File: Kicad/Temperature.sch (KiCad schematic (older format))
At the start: 2 parts

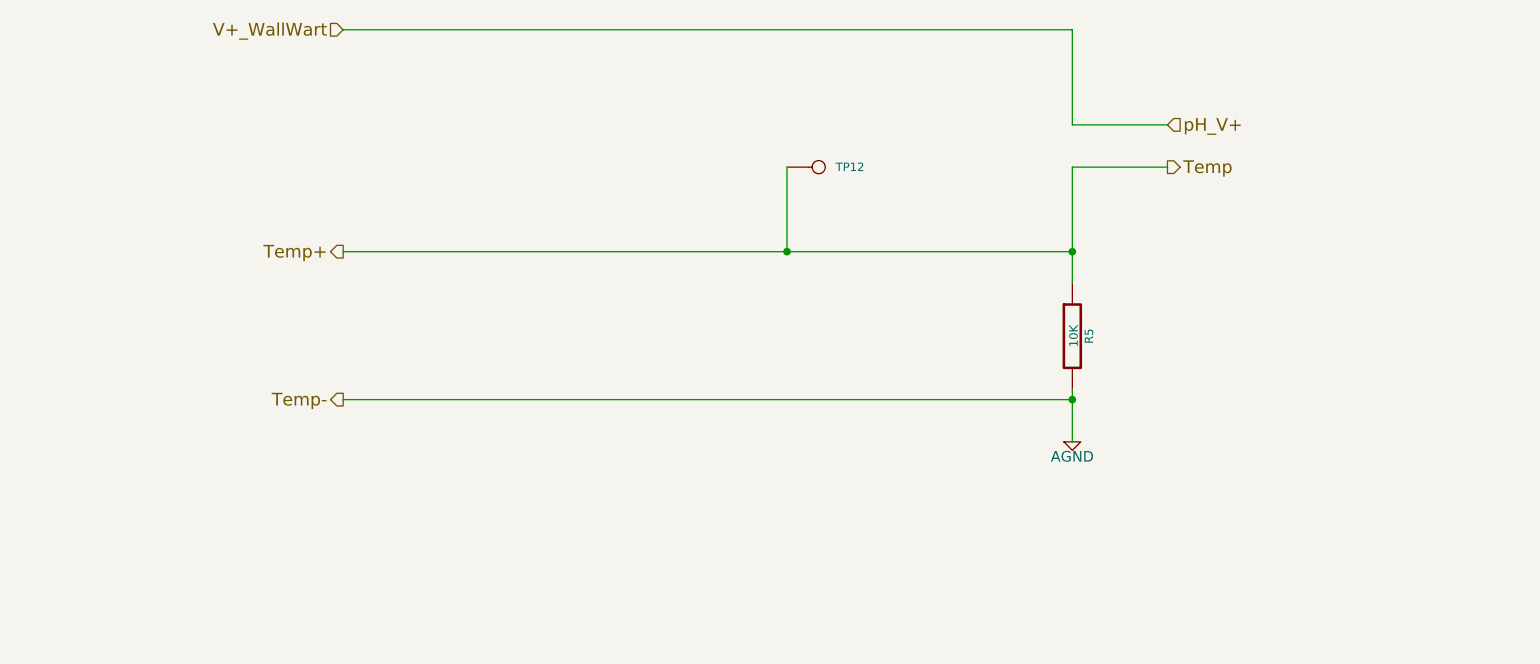
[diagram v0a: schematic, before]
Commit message: updates for dev rev 2
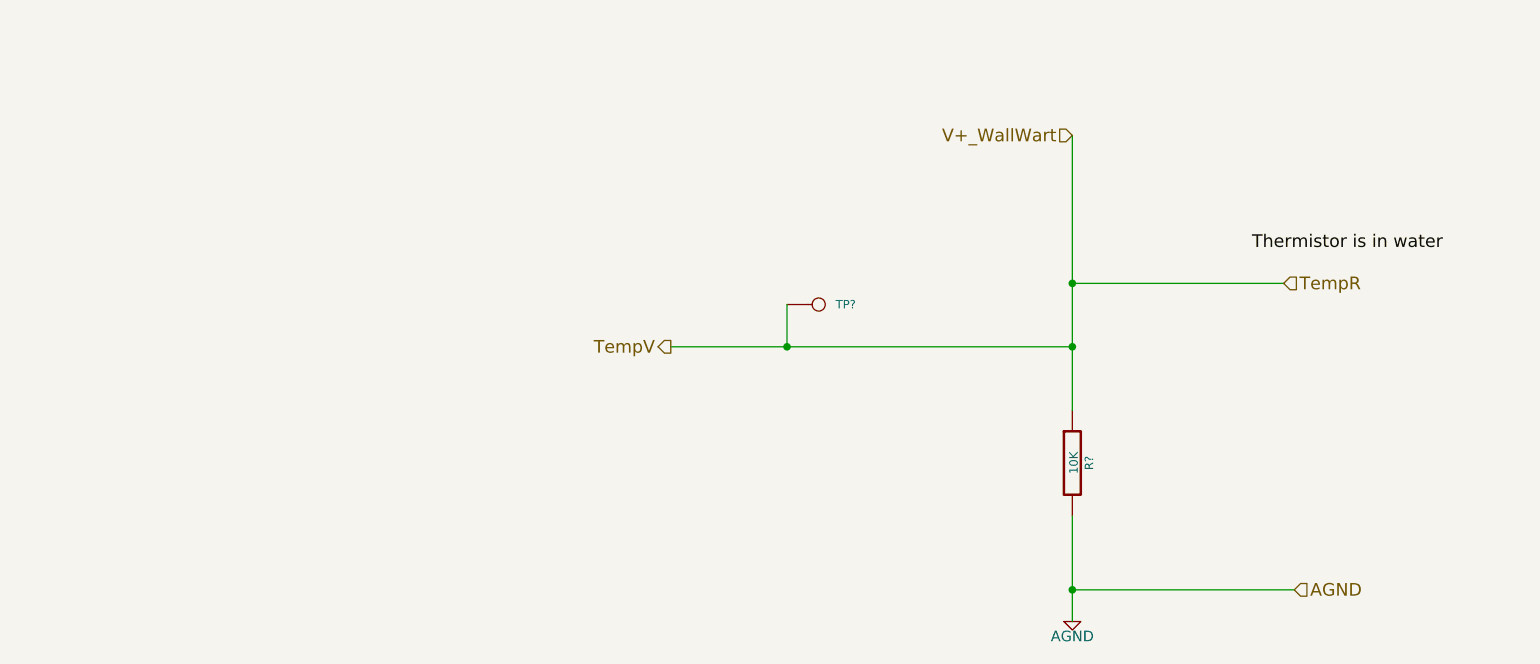
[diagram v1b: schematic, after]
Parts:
- removed R5: 10K, ~, symbol R
- removed TP12: CONN_1, symbol CONN_1
- added R?: 10K, ~, symbol R
- added TP?: CONN_1, symbol CONN_1
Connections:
- net AGND: now also R?.2
- new net TempR: R?.1, TP?.1
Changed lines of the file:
@@
 Sheet 6 7
 Title ""
-Date "21 aug 2014"
+Date "9 sep 2014"
 Rev ""
 Comp ""
@@
 Comment4 ""
 $EndDescr
-Text HLabel 1950 1500 0    60   Input ~ 0
+Text HLabel 5400 2000 0    60   Input ~ 0
 V+_WallWart
-Wire Wire Line
-	1950 1500 5400 1500
 $Comp
 L AGND #PWR012
 U 1 1 53CE414D
-P 5400 3450
-F 0 "#PWR012" H 5400 3450 40  0001 C CNN
-F 1 "AGND" H 5400 3380 50  0000 C CNN
-F 2 "" H 5400 3450 60  0000 C CNN
-F 3 "" H 5400 3450 60  0000 C CNN
-	1    5400 3450
+P 5400 4300
+F 0 "#PWR012" H 5400 4300 40  0001 C CNN
+F 1 "AGND" H 5400 4230 50  0000 C CNN
+F 2 "" H 5400 4300 60  0000 C CNN
+F 3 "" H 5400 4300 60  0000 C CNN
+	1    5400 4300
+	1    0    0    -1
+$EndComp
+$Comp
+L R R?
+U 1 1 540DEB6D
+P 5400 3550
+F 0 "R?" V 5480 3550 40  0000 C CNN
+F 1 "10K" V 5407 3551 40  0000 C CNN
+F 2 "~" V 5330 3550 30  0000 C CNN
+F 3 "~" H 5400 3550 30  0000 C CNN
+	1    5400 3550
+	1    0    0    -1
+$EndComp
+Text HLabel 6400 2700 2    60   Input ~ 0
+TempR
+Text HLabel 3500 3000 0    60   Output ~ 0
+TempV
+Text HLabel 6450 4150 2    60   Input ~ 0
+AGND
+$Comp
+L CONN_1 TP?
+U 1 1 540E05A9
+P 4200 2800
+F 0 "TP?" H 4280 2800 40  0000 L CNN
+F 1 "CONN_1" H 4200 2855 30  0001 C CNN
+F 2 "" H 4200 2800 60  0000 C CNN
+F 3 "" H 4200 2800 60  0000 C CNN
+	1    4200 2800
 	1    0    0    -1
 $EndComp
 Wire Wire Line
-	5400 1500 5400 1950
-$Comp
-L R R5
-U 1 1 53CE4168
-P 5400 2950
-F 0 "R5" V 5480 2950 40  0000 C CNN
-F 1 "10K" V 5407 2951 40  0000 C CNN
-F 2 "~" V 5330 2950 30  0000 C CNN
-F 3 "~" H 5400 2950 30  0000 C CNN
-	1    5400 2950
-	1    0    0    -1
-$EndComp
+	5400 3800 5400 4300
 Wire Wire Line
-	5400 3200 5400 3450
+	5400 2000 5400 3300
 Wire Wire Line
-	5400 2150 5400 2700
+	3500 3000 5400 3000
 Wire Wire Line
-	1950 2550 5400 2550
-Connection ~ 5400 2550
-Text HLabel 1950 2550 0    60   Output ~ 0
-Temp+
-Text HLabel 1950 3250 0    60   Output ~ 0
-Temp-
+	5400 4150 6450 4150
+Connection ~ 5400 4150
 Wire Wire Line
-	1950 3250 5400 3250
-Connection ~ 5400 3250
+	4050 3000 4050 2800
+Connection ~ 5400 3000
+Connection ~ 4050 3000
 Wire Wire Line
-	5850 2150 5400 2150
-Wire Wire Line
-	5400 1950 5850 1950
-Text HLabel 5850 1950 2    60   Input ~ 0
-pH_V+
-Text HLabel 5850 2150 2    60   Output ~ 0
-Temp
-$Comp
-L CONN_1 TP12
-U 1 1 53F5F81F
-P 4200 2150
-F 0 "TP12" H 4280 2150 40  0000 L CNN
-F 1 "CONN_1" H 4200 2205 30  0001 C CNN
-F 2 "" H 4200 2150 60  0000 C CNN
-F 3 "" H 4200 2150 60  0000 C CNN
-	1    4200 2150
-	1    0    0    -1
-$EndComp
-Wire Wire Line
-	4050 2150 4050 2550
-Connection ~ 4050 2550
+	6400 2700 5400 2700
+Connection ~ 5400 2700
+Text Label 6250 2550 0    60   ~ 0
+Thermistor is in water
 $EndSCHEMATC

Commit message: Ready for Schematic Design Review
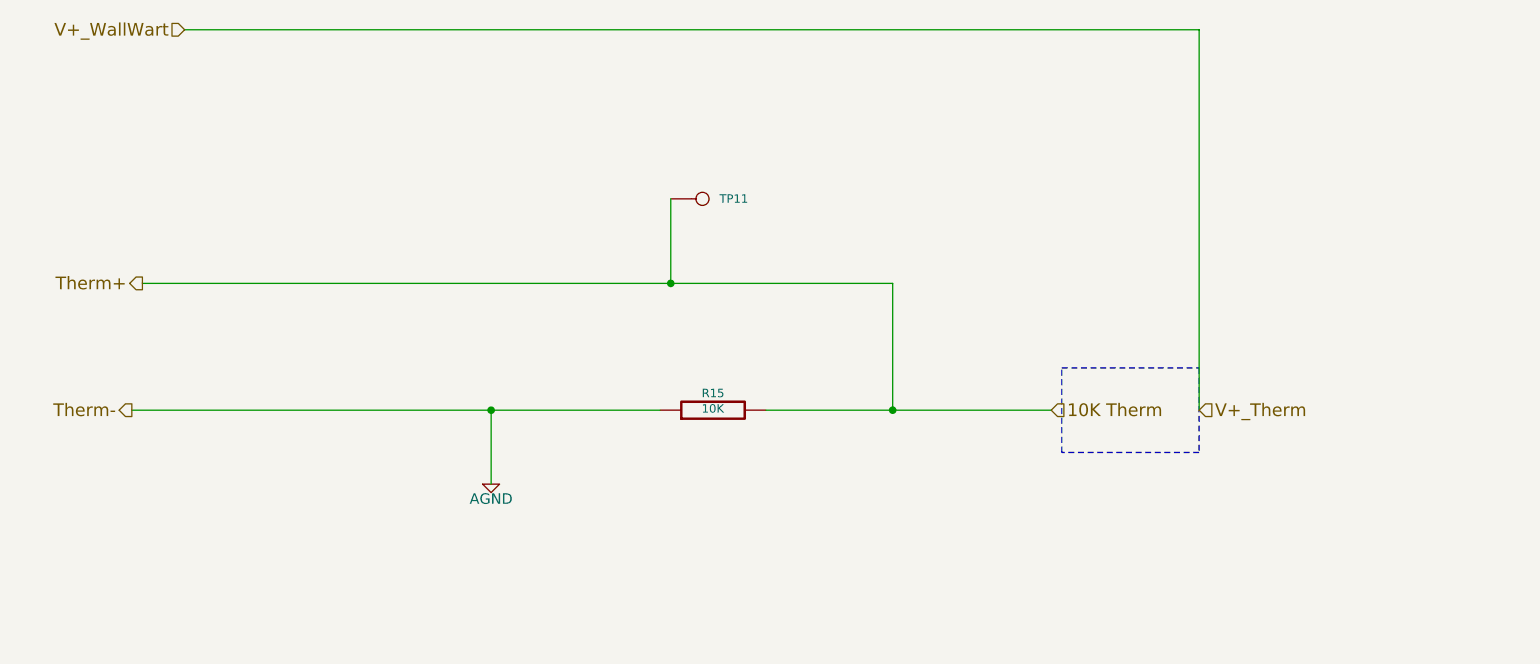
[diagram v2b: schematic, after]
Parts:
- gave numbers to parts that had none: 2
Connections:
- net AGND: now also R15.1; no longer R15.2
- net TempR renamed 10K Therm
- net 10K Therm: now also R15.2; no longer R15.1
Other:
- moved on the sheet: R15, TP11
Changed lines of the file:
@@
 $Descr A4 11693 8268
 encoding utf-8
-Sheet 6 7
+Sheet 4 7
 Title ""
-Date "9 sep 2014"
+Date "10 sep 2014"
 Rev ""
 Comp ""
@@
 Comment4 ""
 $EndDescr
-Text HLabel 5400 2000 0    60   Input ~ 0
-V+_WallWart
+Text HLabel 6000 3300 2    60   Input ~ 0
+V+_Therm
 $Comp
-L AGND #PWR012
+L AGND #PWR04
 U 1 1 53CE414D
-P 5400 4300
-F 0 "#PWR012" H 5400 4300 40  0001 C CNN
-F 1 "AGND" H 5400 4230 50  0000 C CNN
-F 2 "" H 5400 4300 60  0000 C CNN
-F 3 "" H 5400 4300 60  0000 C CNN
-	1    5400 4300
+P 2650 3650
+F 0 "#PWR04" H 2650 3650 40  0001 C CNN
+F 1 "AGND" H 2650 3580 50  0000 C CNN
+F 2 "" H 2650 3650 60  0000 C CNN
+F 3 "" H 2650 3650 60  0000 C CNN
+	1    2650 3650
 	1    0    0    -1
 $EndComp
 $Comp
-L R R?
+L R R15
 U 1 1 540DEB6D
-P 5400 3550
-F 0 "R?" V 5480 3550 40  0000 C CNN
-F 1 "10K" V 5407 3551 40  0000 C CNN
-F 2 "~" V 5330 3550 30  0000 C CNN
-F 3 "~" H 5400 3550 30  0000 C CNN
-	1    5400 3550
-	1    0    0    -1
+P 3700 3300
+F 0 "R15" V 3780 3300 40  0000 C CNN
+F 1 "10K" V 3707 3301 40  0000 C CNN
+F 2 "~" V 3630 3300 30  0000 C CNN
+F 3 "~" H 3700 3300 30  0000 C CNN
+	1    3700 3300
+	0    -1   -1   0
 $EndComp
-Text HLabel 6400 2700 2    60   Input ~ 0
-TempR
-Text HLabel 3500 3000 0    60   Output ~ 0
-TempV
-Text HLabel 6450 4150 2    60   Input ~ 0
-AGND
+Text HLabel 5300 3300 2    60   Input ~ 0
+10K Therm
+Text HLabel 1000 2700 0    60   Output ~ 0
+Therm+
 $Comp
-L CONN_1 TP?
+L CONN_1 TP11
 U 1 1 540E05A9
-P 4200 2800
-F 0 "TP?" H 4280 2800 40  0000 L CNN
-F 1 "CONN_1" H 4200 2855 30  0001 C CNN
-F 2 "" H 4200 2800 60  0000 C CNN
-F 3 "" H 4200 2800 60  0000 C CNN
-	1    4200 2800
+P 3650 2300
+F 0 "TP11" H 3730 2300 40  0000 L CNN
+F 1 "CONN_1" H 3650 2355 30  0001 C CNN
+F 2 "" H 3650 2300 60  0000 C CNN
+F 3 "" H 3650 2300 60  0000 C CNN
+	1    3650 2300
 	1    0    0    -1
 $EndComp
 Wire Wire Line
-	5400 3800 5400 4300
+	950  3300 3450 3300
 Wire Wire Line
-	5400 2000 5400 3300
+	2650 3300 2650 3650
 Wire Wire Line
-	3500 3000 5400 3000
+	3950 3300 5300 3300
 Wire Wire Line
-	5400 4150 6450 4150
-Connection ~ 5400 4150
+	1000 2700 4550 2700
 Wire Wire Line
-	4050 3000 4050 2800
-Connection ~ 5400 3000
-Connection ~ 4050 3000
+	4550 2700 4550 3300
+Connection ~ 4550 3300
 Wire Wire Line
-	6400 2700 5400 2700
-Connection ~ 5400 2700
-Text Label 6250 2550 0    60   ~ 0
-Thermistor is in water
+	3500 2300 3500 2700
+Connection ~ 3500 2700
+Wire Notes Line
+	6000 3100 6000 3500
+Wire Notes Line
+	6000 3500 5350 3500
+Wire Notes Line
+	5350 3500 5350 3100
+Wire Notes Line
+	5350 3100 6000 3100
+Text HLabel 1200 1500 0    60   Input ~ 0
+V+_WallWart
+Wire Wire Line
+	6000 3300 6000 1500
+Wire Wire Line
+	6000 1500 1200 1500
+Text HLabel 950  3300 0    60   Output ~ 0
+Therm-
+Connection ~ 2650 3300
 $EndSCHEMATC
